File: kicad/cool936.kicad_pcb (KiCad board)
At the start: 2 copper layers, 260.6 x 193.1 mm, 88 parts, among them J12 MJ-4PP-9, J13 MJ-4PP-9, SW1 Switch_SW_Push, SW10 Switch_SW_Push, SW101 Switch_SW_Push, SW102 Switch_SW_Push, SW103 Switch_SW_Push, SW11 Switch_SW_Push, SW12 Switch_SW_Push, SW13 Switch_SW_Push, SW14 Switch_SW_Push, SW15 Switch_SW_Push, SW16 Switch_SW_Push, SW17 Switch_SW_Push, SW18 Switch_SW_Push, SW19 Switch_SW_Push, SW2 Switch_SW_Push, SW20 Switch_SW_Push, SW201 Switch_SW_Push, SW21 Switch_SW_Push, SW22 Switch_SW_Push, SW23 Switch_SW_Push, SW24 Switch_SW_Push, SW25 Switch_SW_Push, SW26 Switch_SW_Push, SW27 Switch_SW_Push, SW28 Switch_SW_Push, SW29 Switch_SW_Push, SW3 Switch_SW_Push, SW30 Switch_SW_Push, SW301 Switch_SW_Push, SW302 Switch_SW_Push, SW303 Switch_SW_Push, SW4 Switch_SW_Push, SW5 Switch_SW_Push, SW6 Switch_SW_Push, SW7 Switch_SW_Push, SW8 Switch_SW_Push, SW900 SW_PUSH, SW901 SW_PUSH, U1 ProMicro, U2 ProMicro

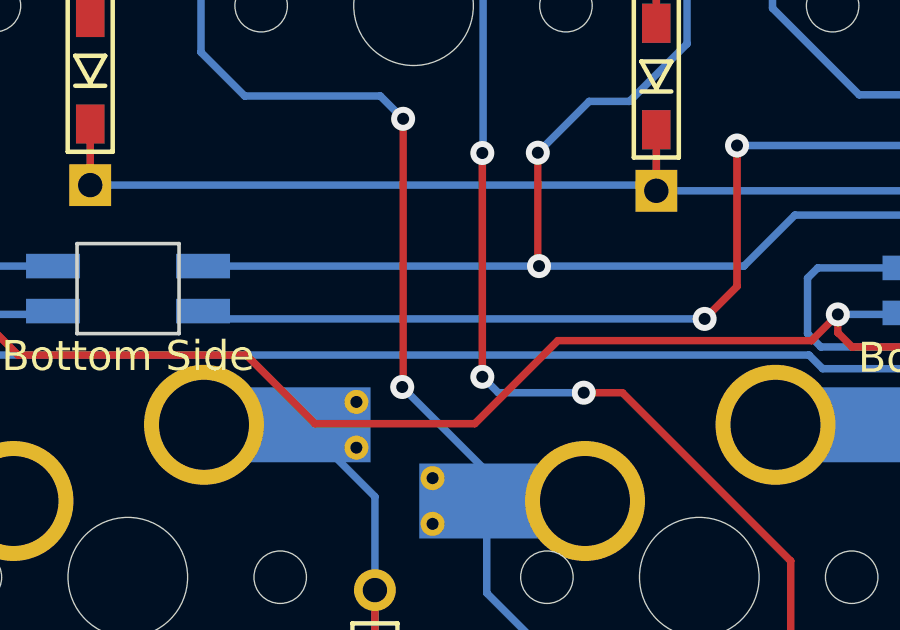
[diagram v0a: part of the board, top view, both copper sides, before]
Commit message: fix
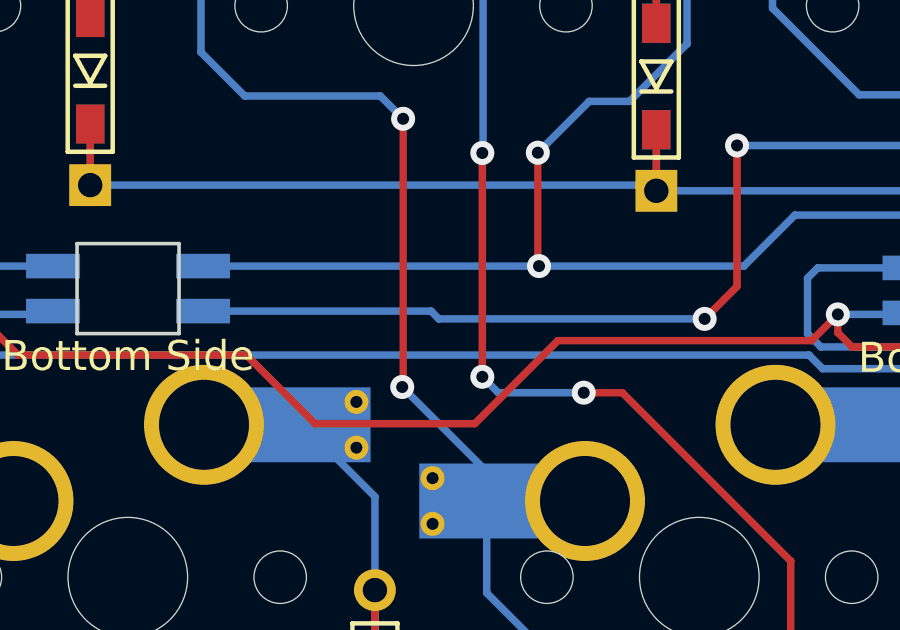
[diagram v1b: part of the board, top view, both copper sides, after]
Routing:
- net LEDR: track 86.8 -> 86.3 mm

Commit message: fix
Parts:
- added J1: Conn_01x03, kbd:StripLED_1side, B.Cu at (113.6, 29.0)
- added J2: Conn_01x03, kbd:StripLED_1side, B.Cu at (190.2, 23.4)
- L1, L2, L3, L4, L5, L6: footprint KiCAD_FootPrint-master:YS-SK6812MINI-E_UG -> kbd:LED_WS2812B-PLCC4
- SW1, SW10, SW101, SW102, SW103, SW11, SW12, SW13, SW14, SW15, SW16, SW17, SW18, SW19, SW2, SW20, SW201, SW21, SW22, SW23, SW24, SW25, SW26, SW27, SW28, SW29, SW3, SW30, SW301, SW302, SW303, SW4, SW5, SW6, SW7, SW8: footprint kbd:CherryMX-Hotswap-v2 -> logo:CherryMX_Hotswap_kimura
- moved D18 18.4 mm to (251.4, 15.5)
- moved G*** 14.9 mm to (71.1, 28.9)
- moved D19 10.0 mm to (267.8, 35.8), turned to 90 degrees
- moved G*** 9.98 mm to (222.4, 30.0)
- moved D11 6.89 mm to (60.8, 14.6)
- moved D102 6.87 mm to (39.4, 14.5)
- moved D12 6.69 mm to (79.7, 14.7)
- moved D17 6.35 mm to (232.6, 16.6)
- moved D16 4.97 mm to (213.5, 16.5)
- moved D15 4.52 mm to (194.3, 16.7)
- moved L4 4.09 mm to (198.4, 25.9)
- moved L2 2.86 mm to (71.5, 25.7)
- moved L3 2.85 mm to (45.1, 25.7)
- moved L1 2.80 mm to (100.0, 25.8)
- moved L6 2.76 mm to (249.7, 25.7)
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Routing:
- net row3R: track 238.8 -> 183.1 mm
- net GND: track 336.4 -> 382.1 mm
- net col3R: track 82.7 -> 108.2 mm
- net VCC: track 291.0 -> 313.9 mm, vias 8 -> 7
- net row1R: track 130.3 -> 147.4 mm
- net Net-(L4-Pad1): track 48.3 -> 32.2 mm, vias 2 -> 0
- net LEDR: track 86.3 -> 102.2 mm, vias 2 -> 1
- net col0R: track 157.0 -> 142.8 mm
- net col2R: track 122.9 -> 113.1 mm
- net row2R: track 147.3 -> 156.7 mm
- net LEDL: track 111.6 -> 120.0 mm, vias 0 -> 2
- net Net-(L5-Pad1): track 40.8 -> 32.6 mm
- net Net-(D18-Pad2): track 30.4 -> 22.4 mm
- net Net-(D26-Pad2): track 17.2 -> 9.75 mm
- net col1R: track 134.9 -> 128.3 mm
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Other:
- board text added: "cool936 designed by m.ki date 20220503 ver.1.3"
- board text removed: "cool936 designed by m.ki date 20220306 ver.1.1"
